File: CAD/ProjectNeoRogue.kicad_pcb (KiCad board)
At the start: 4 copper layers, 95.5 x 113.7 mm, 95 parts, among them J1 5v GND, J10 Conn_01x01_Socket, J2 Micro_SD_Card, J3 JTAG, J4 UART, J5 Reset Jumper, J6 Boot Jumper, J7 RoundDisplay_SPI, J8 USB_C_Plug_USB2.0, J9 RoundDisplay_SPI_v2, SW1 On/Off, SW10 RotaryEncoder_Switch, SW2 Boot, SW3 Reset, SW9 RotaryEncoder_Switch, U1 LTC4054, U2 ESP32-S3-WROOM-1, U3 CH340N, U4 TLV1117LV33, U5 MAX17048, X1 sao_v169bis

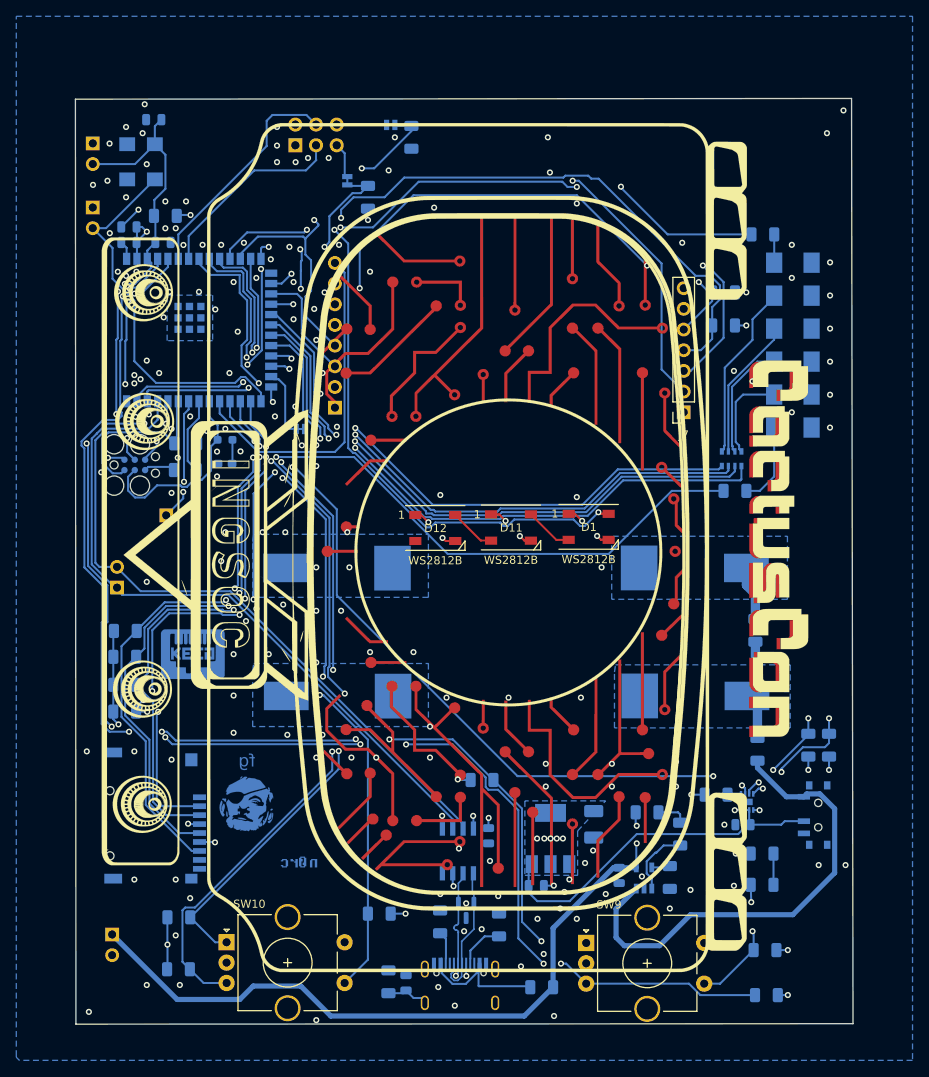
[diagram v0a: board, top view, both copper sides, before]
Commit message: adding art
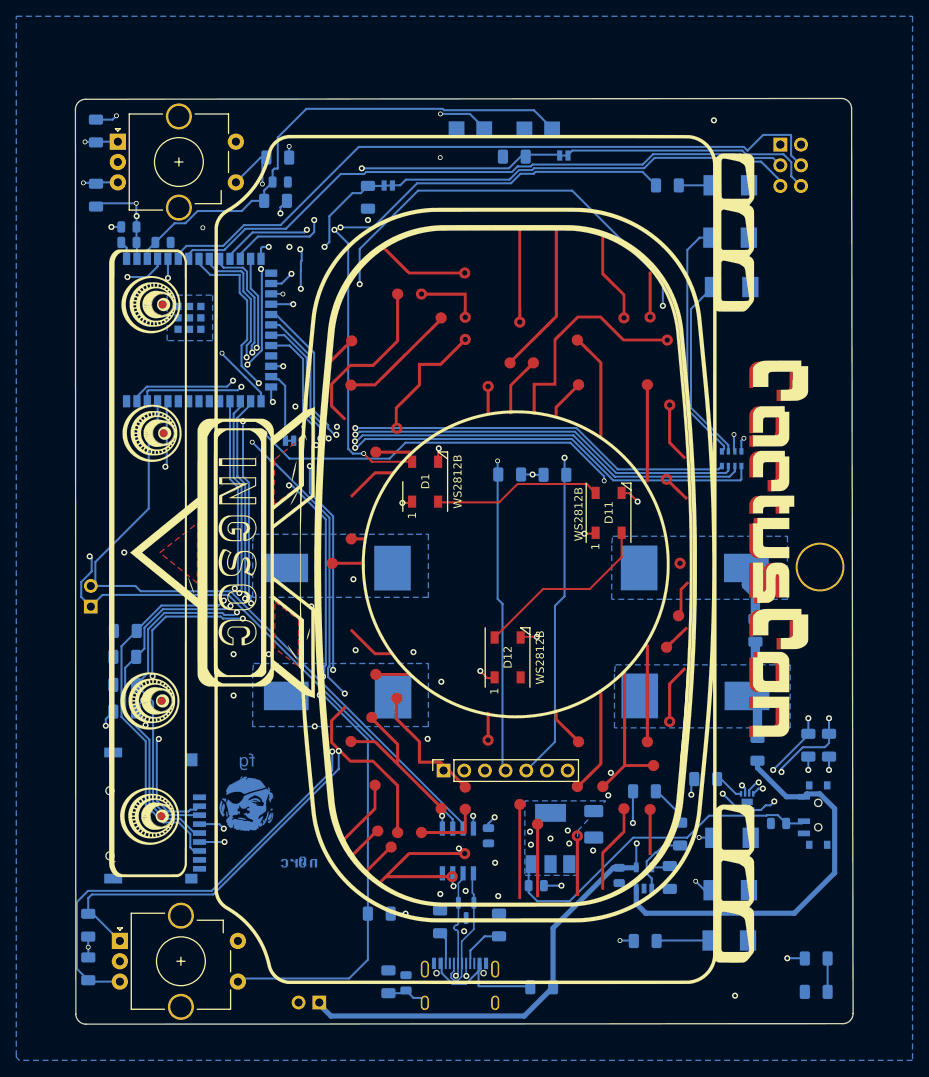
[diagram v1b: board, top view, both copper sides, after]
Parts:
- removed C11: 100pF, Capacitor_SMD:C_0603_1608Metric_Pad1.08x0.95mm_HandSolder
- removed the G*** at (137.1, 113.8)
- removed J10: Conn_01x01_Socket, Connector_PinHeader_2.54mm:PinHeader_1x01_P2.54mm_Vertical
- removed J3: JTAG, Connector:Tag-Connect_TC2030-IDC-FP_2x03_P1.27mm_Vertical
- removed J5: Reset Jumper, BadgePirates:PinHeader_1x02_P2.54mm_Vertical
- removed J6: Boot Jumper, BadgePirates:PinHeader_1x02_P2.54mm_Vertical
- removed J9: RoundDisplay_SPI_v2, Connector_PinSocket_2.54mm:PinSocket_1x08_P2.54mm_Vertical
- removed R21: 75k, Resistor_SMD:R_0603_1608Metric_Pad0.98x0.95mm_HandSolder
- removed R22: 10K, BadgePirates:R_1206_3216Metric
- removed R24: 22k, BadgePirates:R_1206_3216Metric
- added REF**: 5.5mm, BadgePirates:Hole_5.5mm, F.Cu at (214.3, 103.3)
- moved R15 128.2 mm to (125.3, 57.6), turned to -90 degrees
- moved R16 114.3 mm to (147.7, 53.0)
- moved SW9 114.0 mm to (128.0, 51.1)
- moved R14 92.8 mm to (125.3, 49.8), turned to 90 degrees
- moved D8 63.5 mm to (203.1, 149.2)
- moved D7 61.4 mm to (203.3, 143.0)
- moved D6 59.0 mm to (203.5, 136.6)
- moved X1 58.7 mm to (210.6, 53.6), turned to -90 degrees
- moved R9 56.4 mm to (192.8, 149.3)
- moved J7 53.0 mm to (168.0, 128.3), turned to 90 degrees
- moved SW3 48.8 mm to (179.7, 49.5)
- moved SW2 40.9 mm to (171.3, 49.4)
- moved R23 32.0 mm to (176.2, 92.0)
- moved R27 30.5 mm to (181.7, 92.0), turned to 0 degrees
- moved J1 26.8 mm to (152.8, 156.8), turned to 90 degrees
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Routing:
- net IO05: track 166.2 -> 22.8 mm, vias 10 -> 2
- net IO20: track 135.5 -> 19.1 mm, vias 4 -> 2
- net IO04: track 142.8 -> 29.0 mm, vias 7 -> 2
- net Net-(D7-A): track 11.5 -> 61.5 mm, vias 0 -> 2
- net IO01: track 107.7 -> 155.6 mm, vias 4 -> 3
- net Net-(JP3-A): track 3.94 -> 50.5 mm
- net Net-(D6-A): track 14.5 -> 59.7 mm, vias 0 -> 2
- net IO38: track 41.8 -> 0.00 mm
- net IO15: track 94.3 -> 132.6 mm, vias 2 -> 4
- net IO18: track 80.6 -> 50.7 mm
- net VBUS: track 88.8 -> 61.5 mm
- net Net-(JP2-B): track 6.14 -> 31.6 mm
- net TCK: track 24.2 -> 0.00 mm
- net TMS: track 21.5 -> 0.00 mm
- net Net-(D11-DOUT): track 5.70 -> 22.7 mm
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- added copper zone on F.Cu, net (none)
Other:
- outline, holes or cut-outs redrawn
